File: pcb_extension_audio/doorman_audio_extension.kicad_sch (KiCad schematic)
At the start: 35 parts, among them J1 Audio Out, J4 Extension Board Connector, J5 Audio In, U1 ES8388

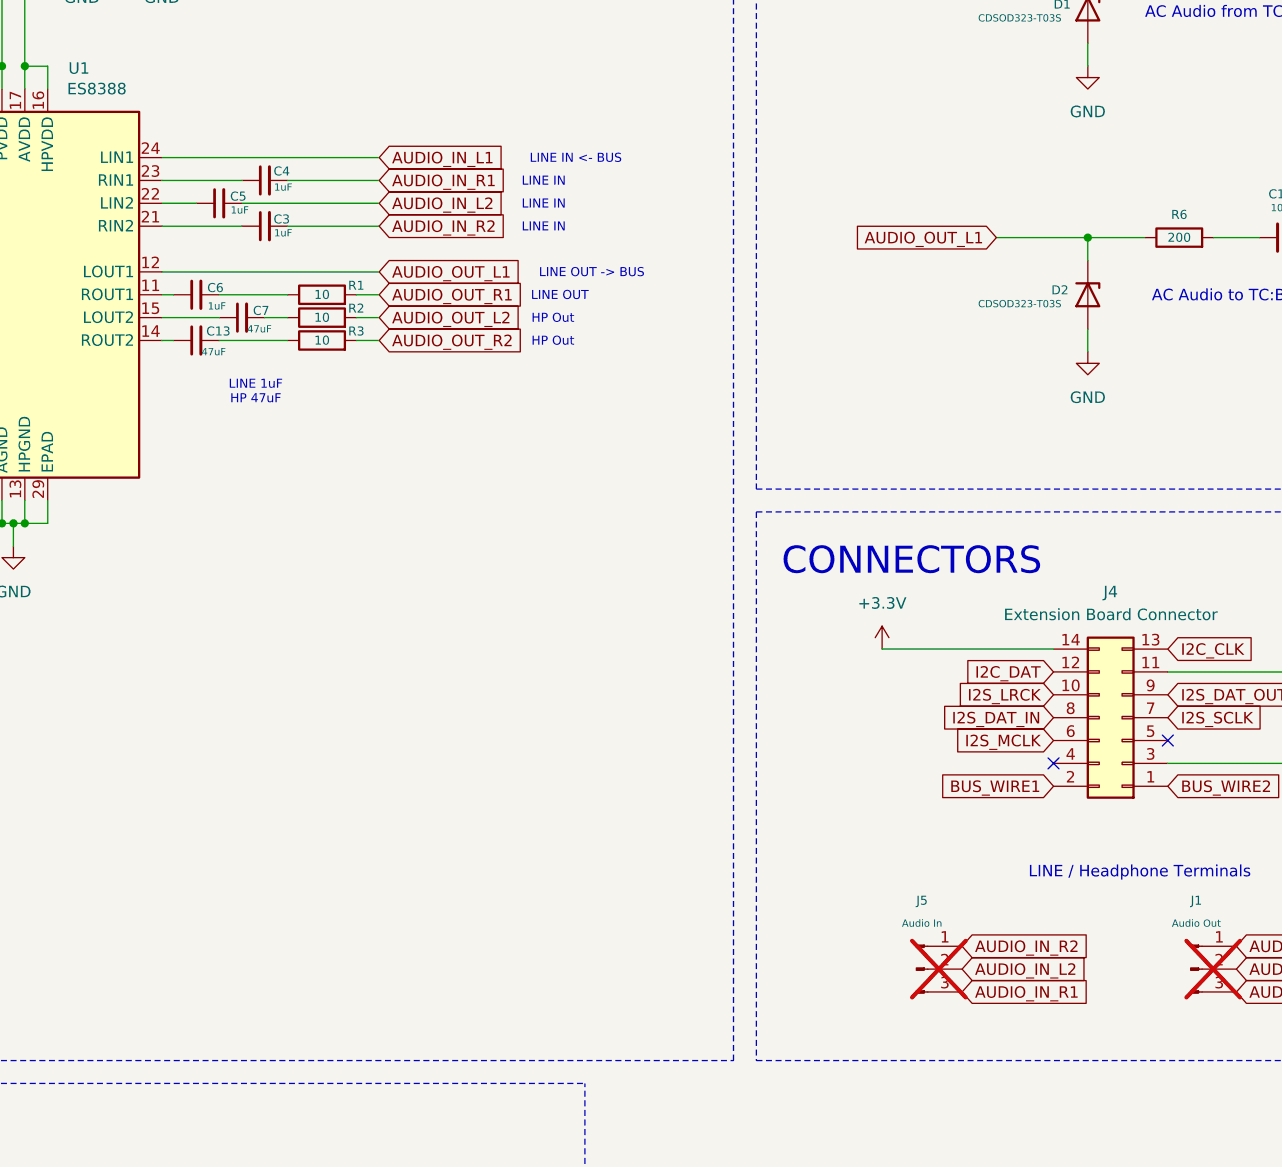
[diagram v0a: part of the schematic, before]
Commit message: WIP
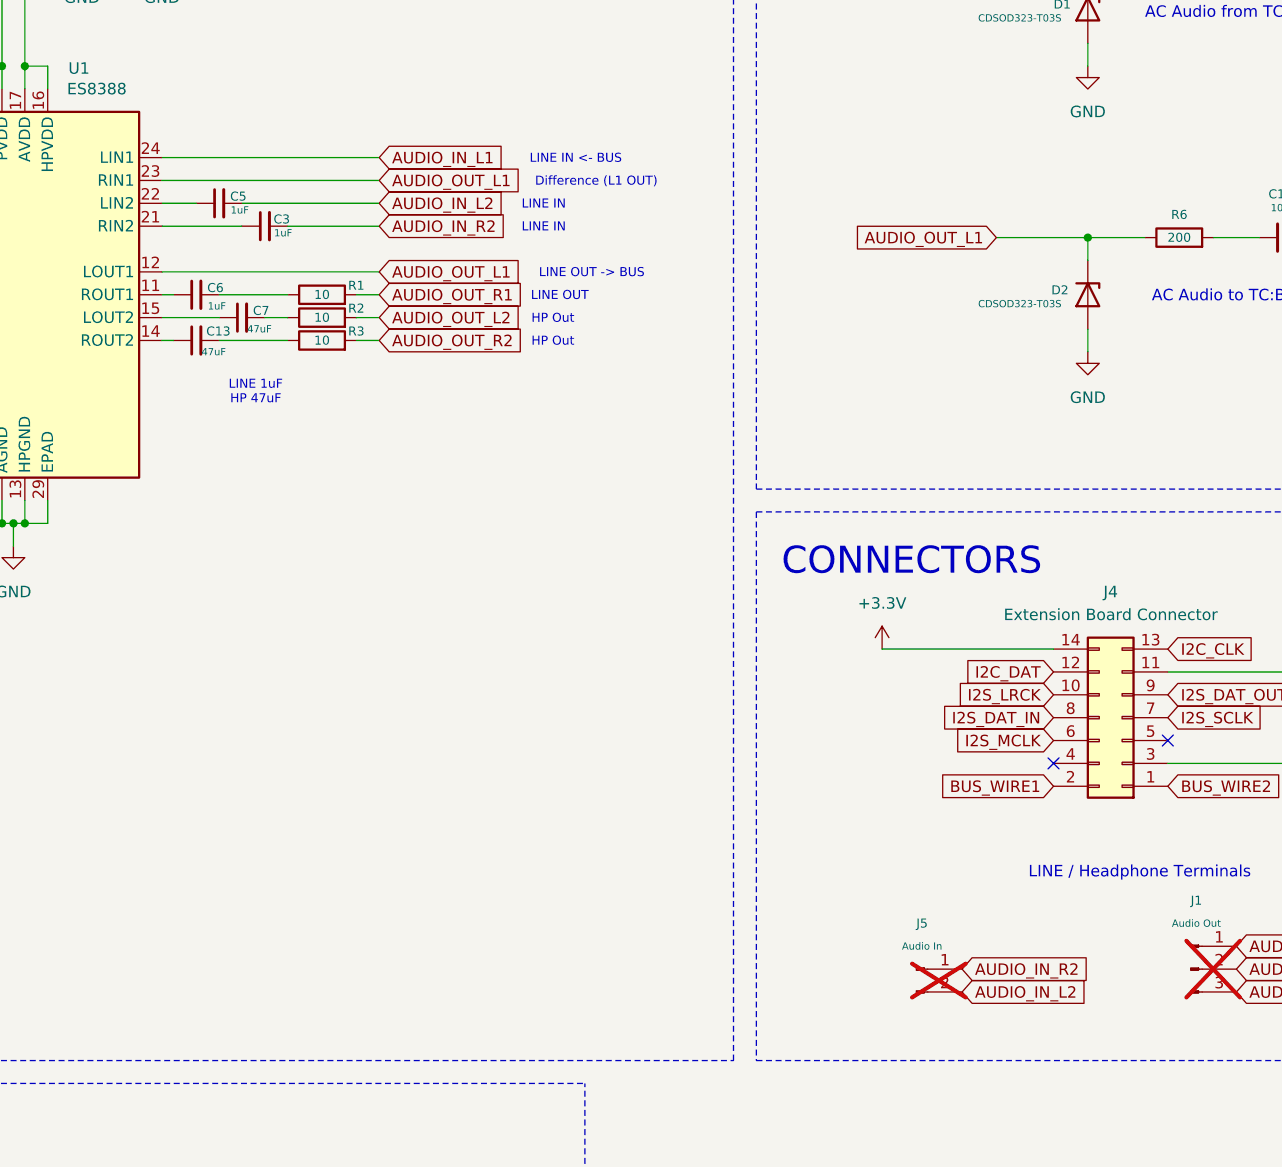
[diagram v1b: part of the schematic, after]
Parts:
- removed C4: 1uF, Capacitor_SMD:C_0603_1608Metric, symbol Device:C_Small
- J5: footprint Connector_PinHeader_2.54mm:PinHeader_1x03_P2.54mm_Vertical -> Connector_PinHeader_2.54mm:PinHeader_1x02_P2.54mm_Vertical; symbol Connector:Conn_01x03_Pin -> Connector:Conn_01x02_Pin
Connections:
- net AUDIO_OUT_L1: now also U1.23 (RIN1)
- removed net AUDIO_IN_R1: J5.3 (Pin_3)
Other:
- note added: "Difference (L1 OUT)"
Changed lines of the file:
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@@
 		)
 	)
+	(text "Difference (L1 OUT)"
+		(exclude_from_sim no)
+		(at 175.26 65.024 0)
+		(effects
+			(font
+				(size 1 1)
+			)
+		)
+	)
 	(text "HP Out"
 		(exclude_from_sim no)
@@
 		)
 	)
-	(text "LINE IN"
-		(exclude_from_sim no)
-		(at 169.418 65.024 0)
-		(effects
-			(font
-				(size 1 1)
-			)
-		)
-	)
 	(text "CONNECTORS"
 		(exclude_from_sim no)
@@
 	(wire
 		(pts
-			(xy 140.97 64.77) (xy 151.13 64.77)
-		)
-		(stroke
-			(width 0)
-			(type default)
-		)
-	)
-	(wire
-		(pts
 			(xy 106.68 100.33) (xy 106.68 102.87)
 		)
@@
 		)
 	)
-	(wire
-		(pts
-			(xy 127 64.77) (xy 135.89 64.77)
-		)
-		(stroke
-			(width 0)
-			(type default)
-		)
-	)
 	(polyline
 		(pts
@@
 	(wire
 		(pts
+			(xy 151.13 64.77) (xy 127 64.77)
+		)
+		(stroke
+			(width 0)
+			(type default)
+		)
+	)
+	(wire
+		(pts
 			(xy 101.6 39.37) (xy 101.6 38.1)
 		)
@@
 		)
 	)
-	(global_label "AUDIO_OUT_R2"
+	(global_label "AUDIO_OUT_L1"
 		(shape input)
-		(at 151.13 82.55 0)
+		(at 151.13 64.77 0)
 		(fields_autoplaced yes)
 		(effects
@@
 		)
 		(property "Intersheetrefs" "${INTERSHEET_REFS}"
-			(at 167.7829 82.55 0)
+			(at 167.541 64.77 0)
 			(effects
 				(font
@@
 		)
 	)
-	(global_label "AUDIO_IN_R2"
+	(global_label "AUDIO_OUT_R2"
 		(shape input)
-		(at 151.13 69.85 0)
+		(at 151.13 82.55 0)
 		(fields_autoplaced yes)
 		(effects
@@
 		)
 		(property "Intersheetrefs" "${INTERSHEET_REFS}"
-			(at 166.0896 69.85 0)
+			(at 167.7829 82.55 0)
 			(effects
 				(font
@@
 		)
 	)
-	(global_label "AUDIO_IN_L2"
+	(global_label "AUDIO_IN_R2"
 		(shape input)
-		(at 215.9 152.4 0)
+		(at 151.13 69.85 0)
 		(fields_autoplaced yes)
 		(effects
@@
 		)
 		(property "Intersheetrefs" "${INTERSHEET_REFS}"
-			(at 230.6177 152.4 0)
+			(at 166.0896 69.85 0)
 			(effects
 				(font
@@
 		)
 	)
-	(global_label "AUDIO_IN_R1"
+	(global_label "AUDIO_IN_L2"
 		(shape input)
-		(at 151.13 64.77 0)
+		(at 215.9 154.94 0)
 		(fields_autoplaced yes)
 		(effects
@@
 		)
 		(property "Intersheetrefs" "${INTERSHEET_REFS}"
-			(at 166.0896 64.77 0)
+			(at 230.6177 154.94 0)
 			(effects
 				(font
@@
 	(global_label "AUDIO_IN_R2"
 		(shape input)
-		(at 215.9 149.86 0)
+		(at 215.9 152.4 0)
 		(fields_autoplaced yes)
 		(effects
@@
 		)
 		(property "Intersheetrefs" "${INTERSHEET_REFS}"
-			(at 230.8596 149.86 0)
+			(at 230.8596 152.4 0)
 			(effects
 				(font
@@
 		)
 	)
-	(global_label "AUDIO_IN_R1"
-		(shape input)
-		(at 215.9 154.94 0)
-		(fields_autoplaced yes)
-		(effects
-			(font
-				(size 1.27 1.27)
-			)
-			(justify left)
-		)
-		(property "Intersheetrefs" "${INTERSHEET_REFS}"
-			(at 230.8596 154.94 0)
-			(effects
-				(font
-					(size 1.27 1.27)
-				)
-				(justify left)
-				(hide yes)
-			)
-		)
-	)
 	(global_label "I2S_SCLK"
 		(shape input)
@@
 	)
 	(symbol
-		(lib_id "Connector:Conn_01x03_Pin")
+		(lib_id "Connector:Conn_01x02_Pin")
 		(at 210.82 152.4 0)
 		(unit 1)
@@
 		(fields_autoplaced yes)
 		(property "Reference" "J5"
-			(at 211.455 144.78 0)
+			(at 211.455 147.32 0)
 			(effects
 				(font
@@
 		)
 		(property "Value" "Audio In"
-			(at 211.455 147.32 0)
+			(at 211.455 149.86 0)
 			(effects
 				(font
@@
 			)
 		)
-		(property "Footprint" "Connector_PinHeader_2.54mm:PinHeader_1x03_P2.54mm_Vertical"
+		(property "Footprint" "Connector_PinHeader_2.54mm:PinHeader_1x02_P2.54mm_Vertical"
 			(at 210.82 152.4 0)
 			(effects
@@
 			)
 		)
-		(property "Description" "Generic connector, single row, 01x03, script generated"
+		(property "Description" "Generic connector, single row, 01x02, script generated"
 			(at 210.82 152.4 0)
 			(effects
@@
 		(pin "2"
 		)
-		(pin "3"
-		)
 		(instances
 			(project "doorman"
@@
 					(unit 1)
 				)
-			)
-		)
-	)
-	(symbol
-		(lib_id "Device:C_Small")
-		(at 138.43 64.77 90)
-		(unit 1)
-		(exclude_from_sim no)
-		(in_bom yes)
-		(on_board yes)
-		(dnp no)
-		(property "Reference" "C4"
-			(at 141.224 63.754 90)
-			(effects
-				(font
-					(size 1 1)
-				)
-				(justify left)
-			)
-		)
-		(property "Value" "1uF"
-			(at 141.478 65.532 90)
-			(effects
-				(font
-					(size 0.8 0.8)
-				)
-				(justify left)
-			)
-		)
-		(property "Footprint" "Capacitor_SMD:C_0603_1608Metric"
-			(at 138.43 64.77 0)
-			(effects
-				(font
-					(size 1.27 1.27)
-				)
-				(hide yes)
-			)
-		)
-		(property "Datasheet" ""
-			(at 138.43 64.77 0)
-			(effects
-				(font
-					(size 1.27 1.27)
-				)
-				(hide yes)
-			)
-		)
-		(property "Description" "1uF 50V X5R ±10% 0603 Multilayer Ceramic Capacitors MLCC - SMD/SMT ROHS"
-			(at 138.43 64.77 0)
-			(effects
-				(font
-					(size 1.27 1.27)
-				)
-				(hide yes)
-			)
-		)
-		(property "LCSC" "C15849"
-			(at 138.43 64.77 0)
-			(effects
-				(font
-					(size 1.27 1.27)
-				)
-				(hide yes)
-			)
-		)
-		(property "MPN" "CL10A105KB8NNNC"
-			(at 138.43 64.77 0)
-			(effects
-				(font
-					(size 1.27 1.27)
-				)
-				(hide yes)
-			)
-		)
-		(property "Height" ""
-			(at 138.43 64.77 0)
-			(effects
-				(font
-					(size 1.27 1.27)
-				)
-				(hide yes)
-			)
-		)
-		(property "Mouser Part Number" ""
-			(at 138.43 64.77 0)
-			(effects
-				(font
-					(size 1.27 1.27)
-				)
-				(hide yes)
-			)
-		)
-		(property "Mouser Price/Stock" ""
-			(at 138.43 64.77 0)
-			(effects
-				(font
-					(size 1.27 1.27)
-				)
-				(hide yes)
-			)
-		)
-		(property "Package" "0603"
-			(at 138.43 64.77 90)
-			(effects
-				(font
-					(size 1.27 1.27)
-				)
-				(hide yes)
-			)
-		)
-		(property "Price" ""
-			(at 138.43 64.77 0)
-			(effects
-				(font
-					(size 1.27 1.27)
-				)
-				(hide yes)
-			)
-		)
-		(property "Cheap Version" ""
-			(at 138.43 64.77 90)
-			(effects
-				(font
-					(size 1.27 1.27)
-				)
-				(hide yes)
-			)
-		)
-		(property "Expensive Version" ""
-			(at 138.43 64.77 90)
-			(effects
-				(font
-					(size 1.27 1.27)
-				)
-				(hide yes)
-			)
-		)
-		(property "LCSC Part" ""
-			(at 138.43 64.77 90)
-			(effects
-				(font
-					(size 1.27 1.27)
-				)
-				(hide yes)
-			)
-		)
-		(property "Manufacturer_Name" ""
-			(at 138.43 64.77 90)
-			(effects
-				(font
-					(size 1.27 1.27)
-				)
-				(hide yes)
-			)
-		)
-		(property "Manufacturer_Part_Number" ""
-			(at 138.43 64.77 90)
-			(effects
-				(font
-					(size 1.27 1.27)
-				)
-				(hide yes)
-			)
-		)
-		(pin "1"
-		)
-		(pin "2"
-		)
-		(instances
-			(project "doorman"
-				(path "/2048a046-8e00-475d-aeec-41a343368725"
-					(reference "C4")
-					(unit 1)
-				)

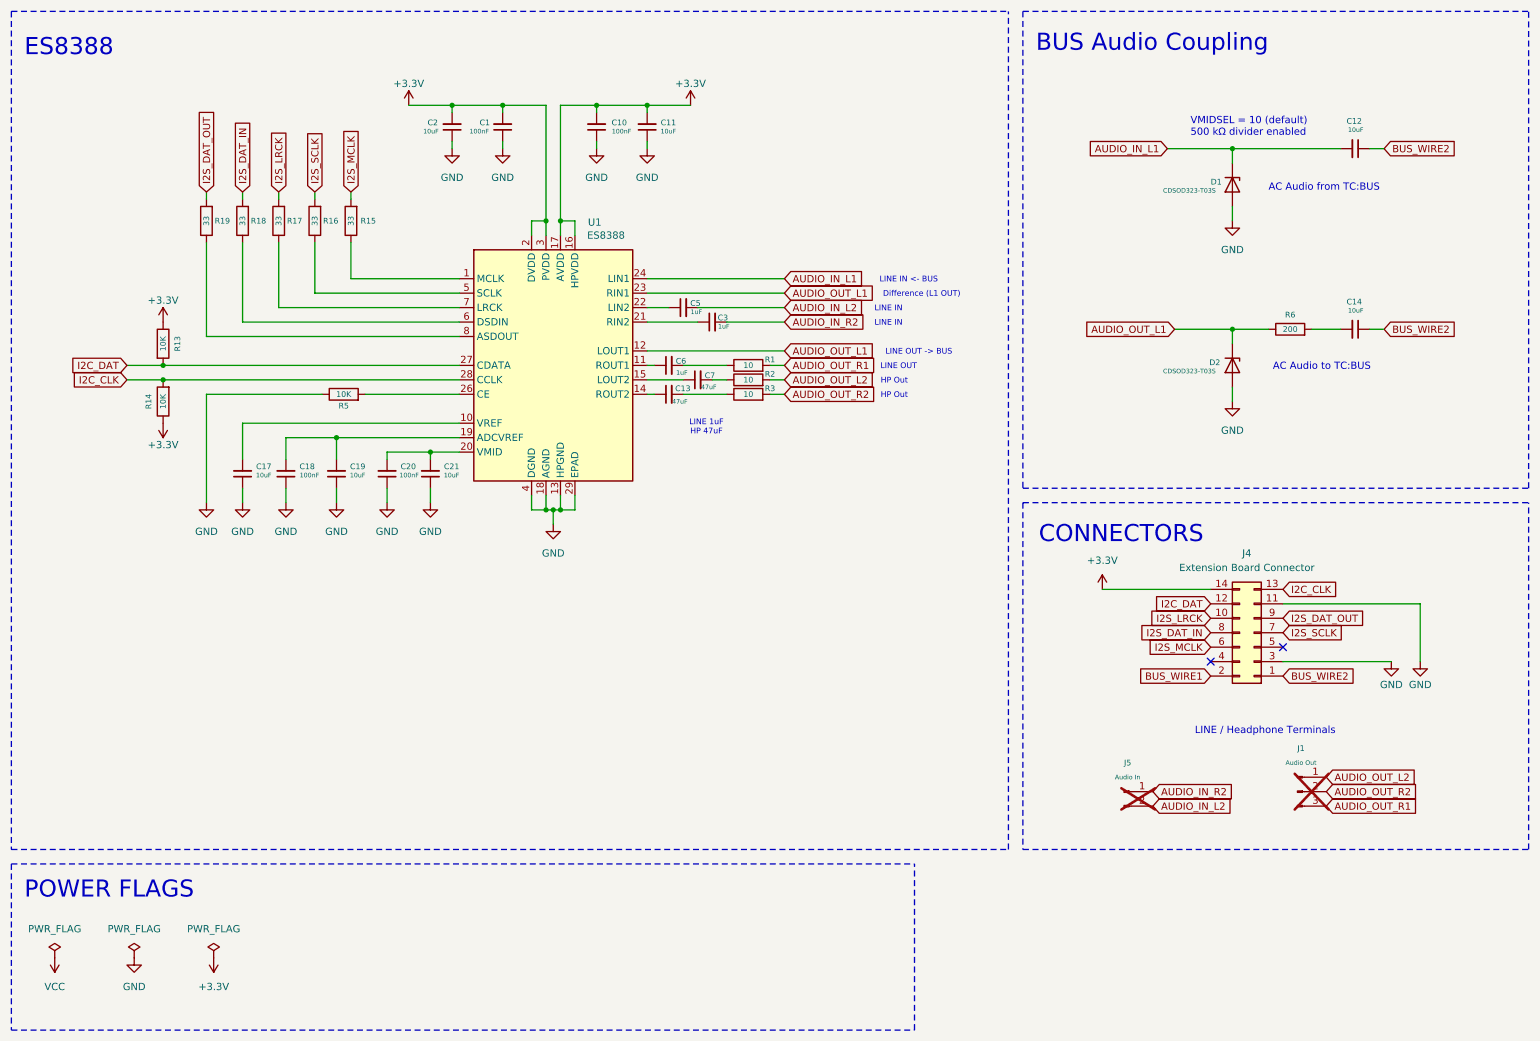
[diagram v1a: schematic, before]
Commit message: WIP
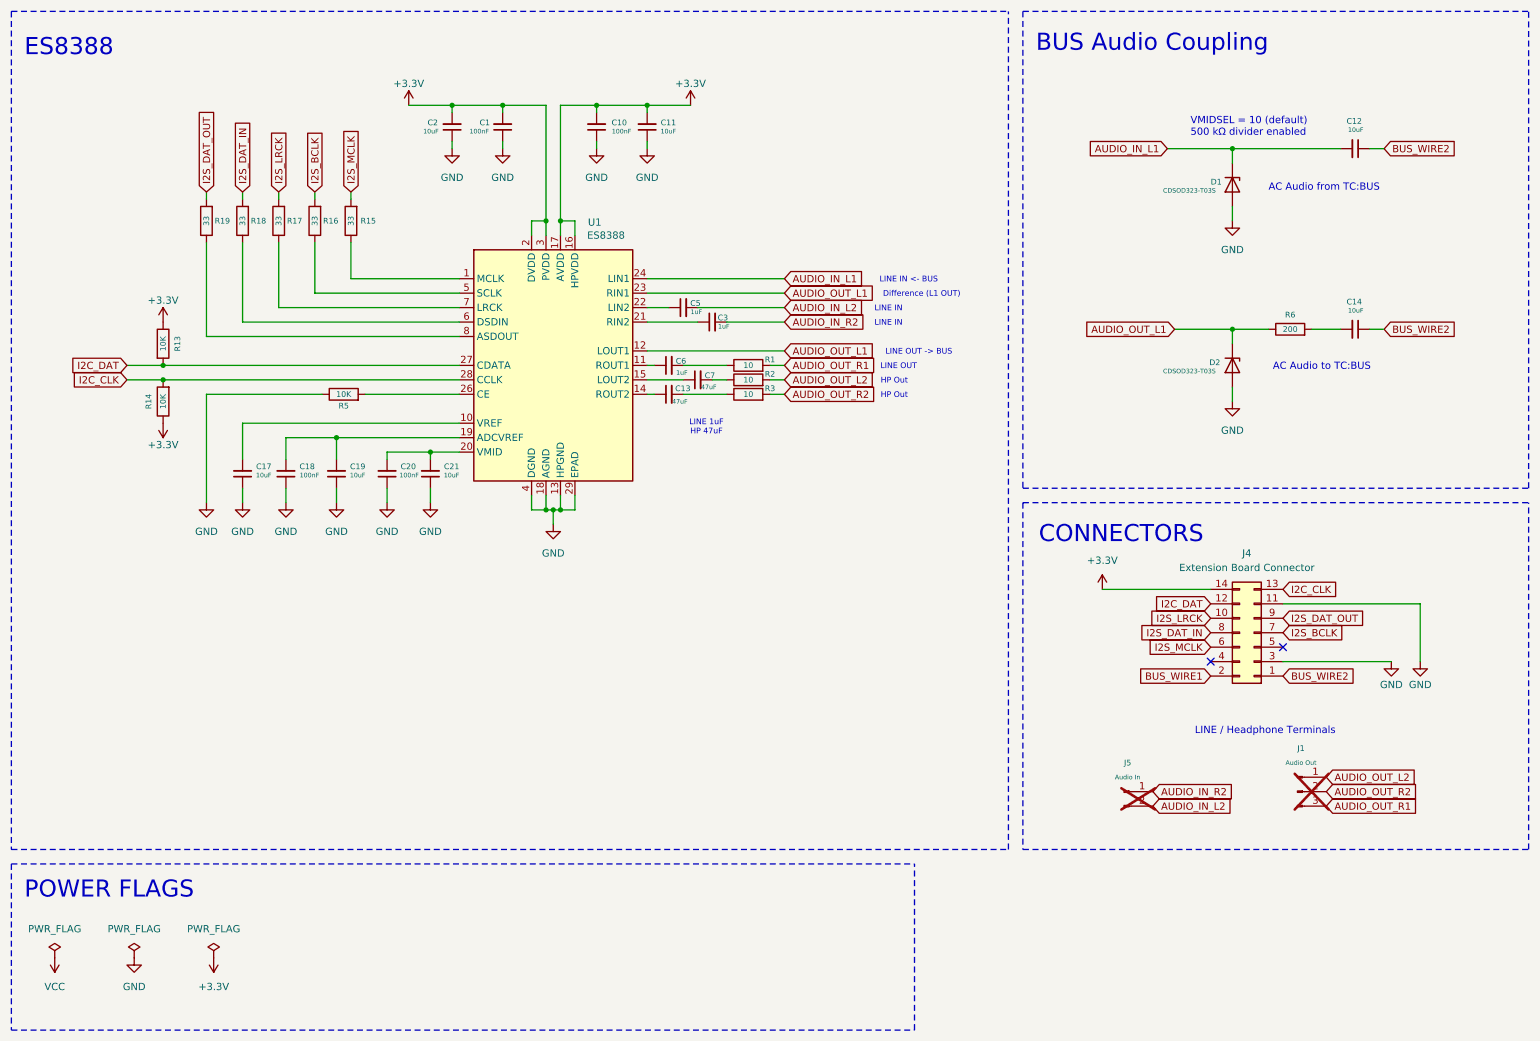
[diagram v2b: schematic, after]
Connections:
- net I2S_SCLK renamed I2S_BCLK
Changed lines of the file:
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@@
 		)
 	)
-	(global_label "I2S_SCLK"
+	(global_label "I2S_BCLK"
 		(shape input)
 		(at 68.58 46.99 90)
@@
 		)
 		(property "Intersheetrefs" "${INTERSHEET_REFS}"
-			(at 68.58 35.2358 90)
+			(at 68.58 35.1753 90)
 			(effects
 				(font
@@
 		)
 	)
-	(global_label "I2S_SCLK"
+	(global_label "I2S_BCLK"
 		(shape input)
 		(at 238.76 124.46 0)
@@
 		)
 		(property "Intersheetrefs" "${INTERSHEET_REFS}"
-			(at 249.3652 124.46 0)
+			(at 250.5747 124.46 0)
 			(effects
 				(font
